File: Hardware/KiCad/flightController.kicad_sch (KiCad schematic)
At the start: 0 parts

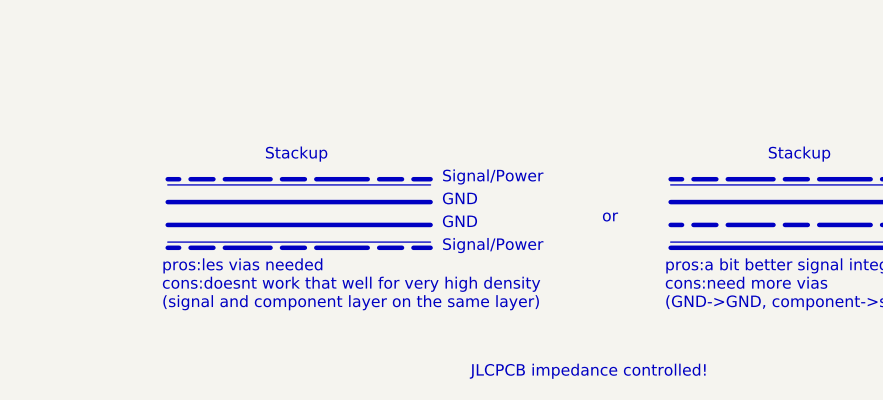
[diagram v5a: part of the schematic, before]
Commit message: Almost finished all routing
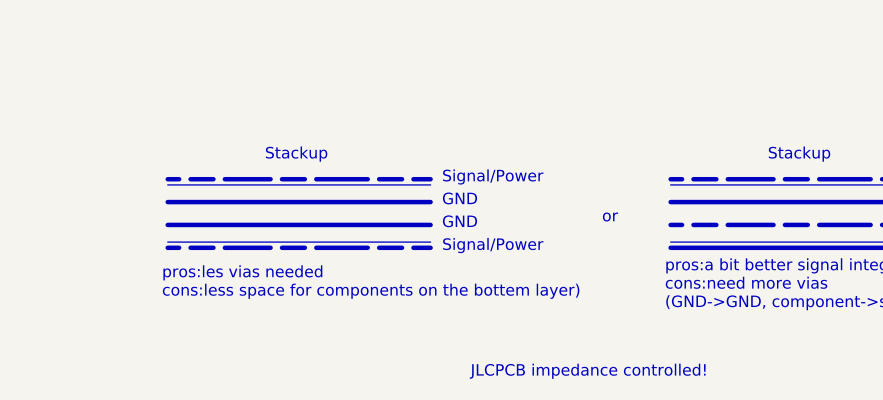
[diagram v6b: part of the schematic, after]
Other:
- note added: "pros:les vias needed cons:less space for components on the bottem layer)"
- note removed: "pros:les vias needed cons:doesnt work that well for very high density (signal and component layer on the same layer)"
